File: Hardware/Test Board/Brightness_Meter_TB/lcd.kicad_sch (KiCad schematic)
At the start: 3 parts, among them U6 SSD1306

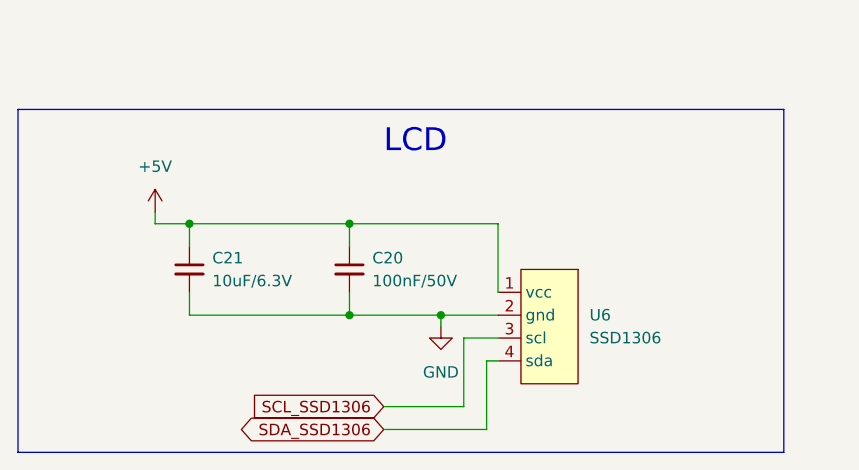
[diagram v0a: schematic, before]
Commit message: upload hardware
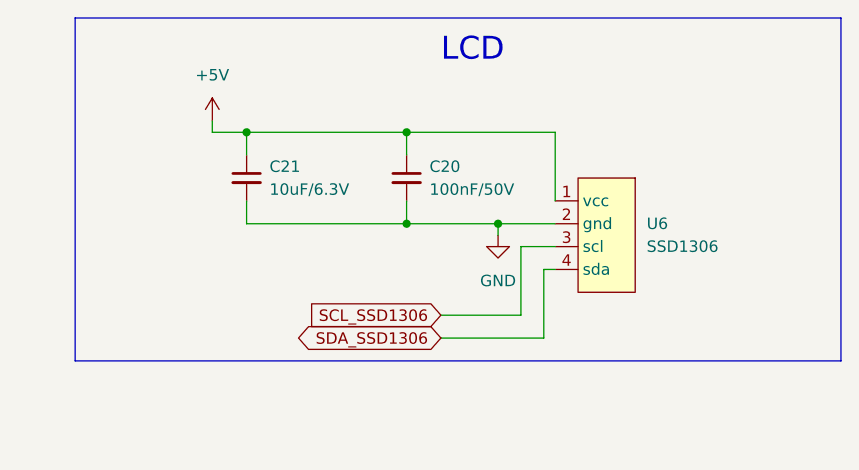
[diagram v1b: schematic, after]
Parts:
- C20, C21: footprint Capacitor_SMD:C_0603_1608Metric_Pad1.08x0.95mm_HandSolder -> Capacitor_SMD:C_0805_2012Metric_Pad1.18x1.45mm_HandSolder
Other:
- title: LCD -> (none)
